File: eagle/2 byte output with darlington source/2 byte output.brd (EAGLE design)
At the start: 85.1 x 44.1 mm, 26 parts, among them IC1 74LS165N, IC2 74LS165N, X1 MKDSN1,5/5-5,08, X2 MKDSN1,5/5-5,08, X3 MKDSN1,5/8-5,08, X5 MKDSN1,5/8-5,08

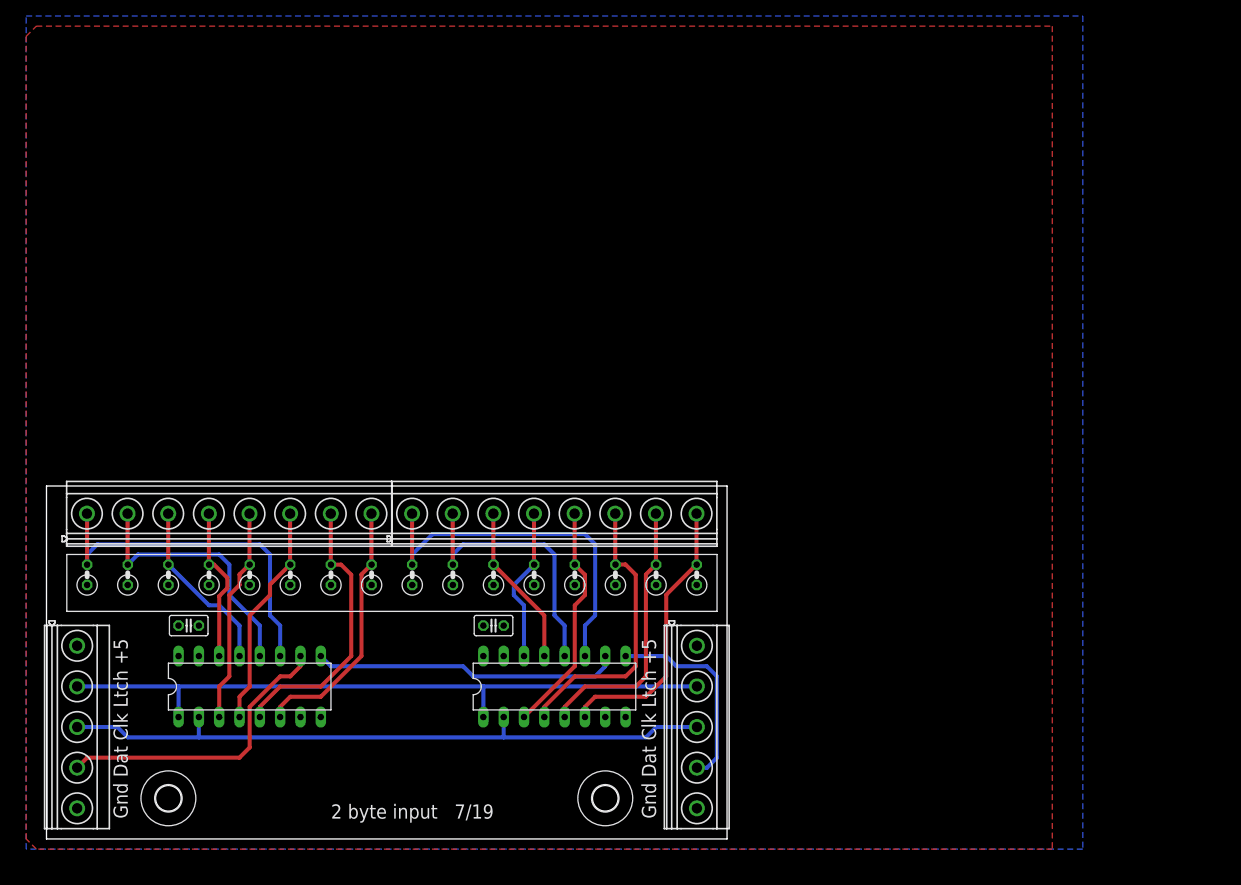
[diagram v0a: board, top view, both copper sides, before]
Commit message: check in changes
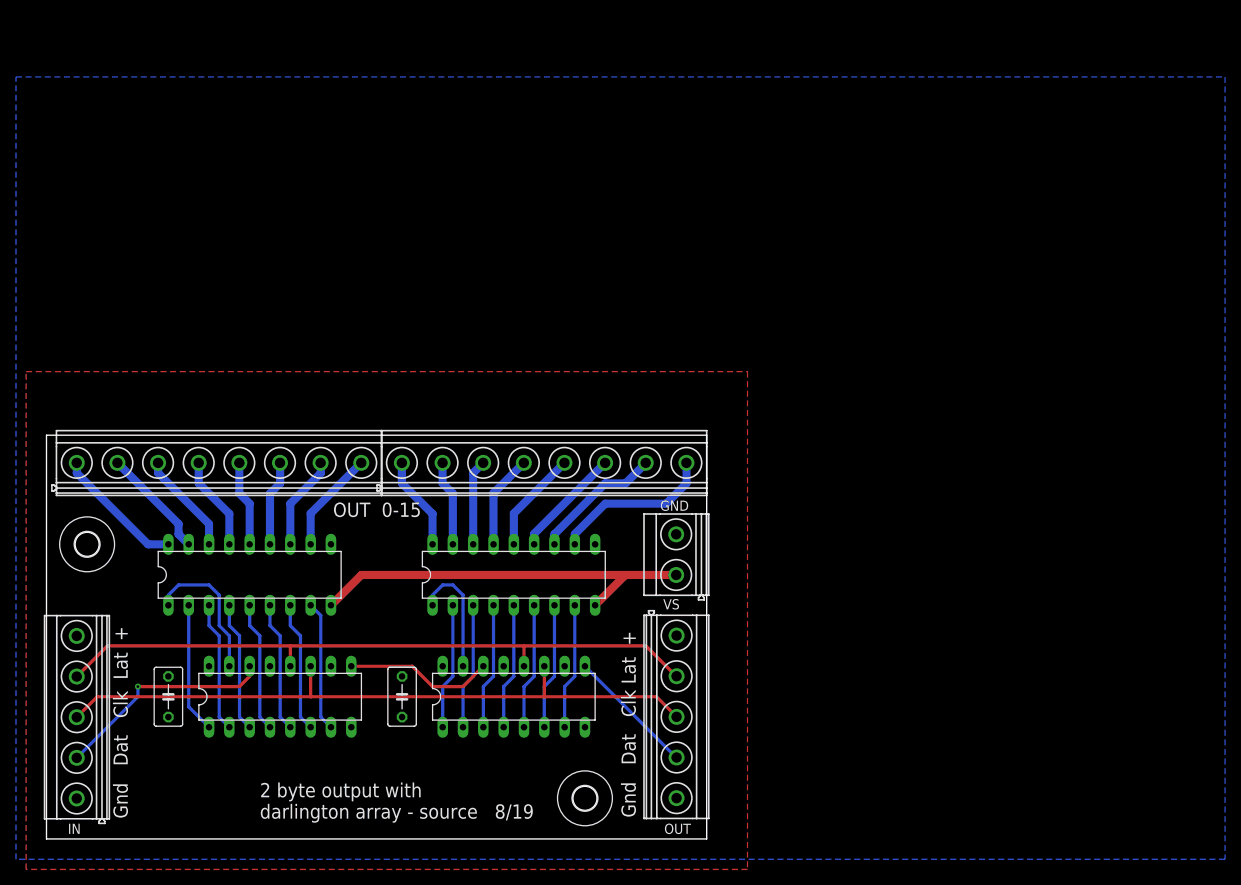
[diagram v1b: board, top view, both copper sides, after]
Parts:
- removed R1, R10, R11, R12, R13, R14, R15, R16, R2, R3, R4, R5, R6, R7, R8: (no value), resistor:0207/2V
- removed R9: 10K, resistor:0207/2V
- added IC3, IC4: UDN2981A, uln-udn:DIL18
- added X4: MKDSN1,5/5-5,08, con-phoenix-508:MKDSN1,5/5-5,08
- C1, C2: value 0.1uf -> (none); device resistor:C025-025X050 -> resistor:C050-035X075
- H1, H2: value MOUNT-HOLE3.2 -> MOUNT-HOLE3.0; device holes:3,2 -> holes:3,0
- IC1, IC2: value 74LS165N -> 74LS595N
- X1, X2: value MKDSN1,5/5-5,08 -> MKDSN1,5/8-5,08; device con-phoenix-508:MKDSN1,5/5-5,08 -> con-phoenix-508:MKDSN1,5/8-5,08
- X3: value MKDSN1,5/8-5,08 -> MKDSN1,5/5-5,08; device con-phoenix-508:MKDSN1,5/8-5,08 -> con-phoenix-508:MKDSN1,5/5-5,08
- X5: value MKDSN1,5/8-5,08 -> MKDSN1,5/2-5,08; device con-phoenix-508:MKDSN1,5/8-5,08 -> con-phoenix-508:MKDSN1,5/2-5,08
- moved X2 38.1 mm to (62.2, 47.0), turned to 0 degrees
- moved X1 37.5 mm to (21.6, 47.0), turned to 0 degrees
- moved H1 33.3 mm to (5.08, 36.8)
- moved X3 31.8 mm to (3.81, 15.2), turned to 90 degrees
- moved X5 16.1 mm to (78.7, 35.6), turned to 90 degrees
- moved C2 14.5 mm to (44.5, 17.8), turned to 270 degrees
- moved C1 9.25 mm to (15.2, 17.8), turned to 270 degrees
- moved IC2 5.24 mm to (58.4, 17.8)
- moved IC1 4.02 mm to (29.2, 17.8)
- moved H2 2.54 mm to (67.3, 5.08)
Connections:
- removed net +5V: C1.1, C2.1, IC1.16, IC2.16, R1.1, R10.1, R11.1, R12.1, R13.1, R14.1, R15.1, R16.1, R2.1, R3.1, R4.1, R5.1, R6.1, R7.1, R8.1, R9.1, X1.1, X2.1
- removed net INA0: IC1.11, R1.2, X3.1
- removed net INA1: IC1.12, R2.2, X3.2
- removed net INA2: IC1.13, R3.2, X3.3
- removed net INA3: IC1.14, R4.2, X3.4
- removed net INA4: IC1.3, R5.2, X3.5
- removed net INA5: IC1.4, R6.2, X3.6
- removed net INA6: IC1.5, R7.2, X3.7
- removed net INA7: IC1.6, R8.2, X3.8
- removed net INB0: IC2.11, R9.2, X5.1
- removed net INB1: IC2.12, R10.2, X5.2
- removed net INB2: IC2.13, R11.2, X5.3
- removed net INB3: IC2.14, R12.2, X5.4
- removed net INB4: IC2.3, R13.2, X5.5
- removed net INB5: IC2.4, R14.2, X5.6
- removed net INB6: IC2.5, R15.2, X5.7
- removed net INB7: IC2.6, R16.2, X5.8
- removed net SER0: IC1.10, X1.4
- removed net SER1: IC1.9, IC2.10
- removed net SERX: IC2.9, X2.4
- new net DI: IC1.14, X3.2
- new net DO: IC2.9, X4.4
- new net DP: IC1.9, IC2.14
- new net N$1: IC3.15, X1.4
- new net N$10: IC4.16, X2.3
- new net N$11: IC4.17, X2.2
- new net N$12: IC4.18, X2.1
- new net N$13: IC4.14, X2.5
- new net N$14: IC4.13, X2.6
- new net N$15: IC4.12, X2.7
- new net N$16: IC4.11, X2.8
- new net N$17: IC1.15, IC3.1
- new net N$18: IC1.1, IC3.2
- new net N$19: IC1.2, IC3.3
- new net N$2: IC3.16, X1.3
- new net N$20: IC1.3, IC3.4
- new net N$21: IC1.4, IC3.5
- new net N$22: IC1.5, IC3.6
- new net N$23: IC1.6, IC3.7
- new net N$24: IC1.7, IC3.8
- new net N$25: IC2.15, IC4.1
- new net N$26: IC2.1, IC4.2
- new net N$27: IC2.2, IC4.3
- new net N$28: IC2.3, IC4.4
- new net N$29: IC2.4, IC4.5
- new net N$3: IC3.17, X1.2
- new net N$30: IC2.5, IC4.6
- new net N$31: IC2.6, IC4.7
- new net N$32: IC2.7, IC4.8
- new net N$4: IC3.18, X1.1
- new net N$5: IC3.14, X1.5
- new net N$6: IC3.12, X1.7
- new net N$7: IC3.11, X1.8
- new net N$8: IC3.13, X1.6
- new net N$9: IC4.15, X2.4
- new net VCC: C1.1, C2.1, IC1.10, IC1.16, IC2.10, IC2.16, X3.5, X4.1
- new net VS: IC3.9, IC4.9, X5.1
- net CLK: now also IC1.11, IC2.11, X3.3, X4.3; no longer IC1.2, IC2.2, X1.3, X2.3
- net GND: now also IC1.13, IC2.13, IC3.10, IC4.10, X3.1, X4.5, X5.2; no longer IC1.15, IC2.15, X1.5, X2.5
- net LATCH: now also IC1.12, IC2.12, X3.4, X4.2; no longer IC1.1, IC2.1, X1.2, X2.2
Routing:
- net VS: track 0.00 -> 50.1 mm
- net INB0: track 46.6 -> 0.00 mm
- net INA0: track 44.8 -> 0.00 mm
- net SER1: track 38.4 -> 0.00 mm
- net SER0: track 37.4 -> 0.00 mm
- net INB5: track 35.7 -> 0.00 mm
- net INB7: track 35.0 -> 0.00 mm
- net INA6: track 34.9 -> 0.00 mm
- net INB1: track 34.6 -> 0.00 mm
- net INB6: track 33.9 -> 0.00 mm
- net INA1: track 33.1 -> 0.00 mm
- net INA7: track 32.4 -> 0.00 mm
- net INB4: track 29.1 -> 0.00 mm
- net INA5: track 28.1 -> 0.00 mm
- net DI: track 0.00 -> 27.8 mm, vias 0 -> 1
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- added copper zone on layer 1, net VCC
- removed copper zone on layer 1, net +5V
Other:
- board size 85.1 x 44.1 mm -> 82.5 x 50.5 mm
- board text added: "2 byte output with darlington array - source 8/19"
- board text added: "GND"
- board text added: "Gnd Dat Clk Lat +"
- board text added: "IN"
- board text added: "OUT"
- board text added: "OUT 0-15"
- board text added: "VS"
- board text removed: "2 byte input 7/19"
- board text removed: "Gnd Dat Clk Ltch +5"
